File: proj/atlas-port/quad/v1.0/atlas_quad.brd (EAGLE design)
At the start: 104.1 x 95.2 mm, 110 parts, among them J11 PJ-036AH, J12 PJ-036AH, J13 5227161-9, J14 Atlas Stamp, J15 I2C-HEADER, J16 54602-908LF, J17 54602-908LF, J19 5227161-9, J20 Atlas Stamp, J21 I2C-HEADER, J4 5227161-9, J5 Atlas Stamp, J6 I2C-HEADER, J7 5227161-9, J8 Atlas Stamp, J9 I2C-HEADER, U10 ISO1540, U11 MIC4680, U12 PCA9615, U13 RM-3.33.3S, U14 ISO1540, U3 RM-3.33.3S, U4 ISO1540, U5 RM-3.33.3S, U6 ISO1540, U8 LM2937, U9 RM-3.33.3S

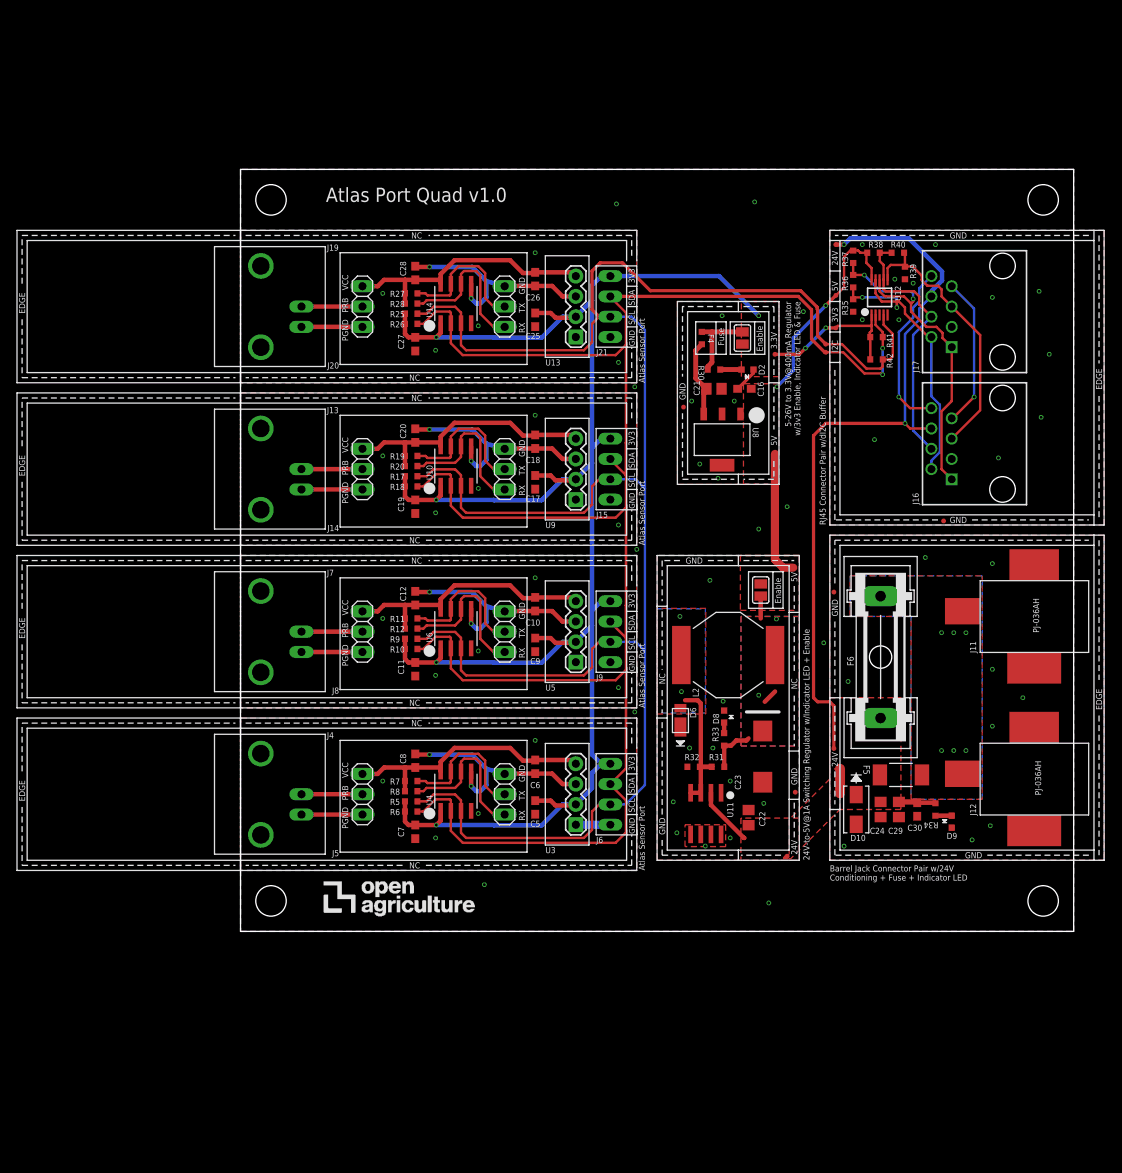
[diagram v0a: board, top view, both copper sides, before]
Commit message: added photon quad v1.0 at 90%
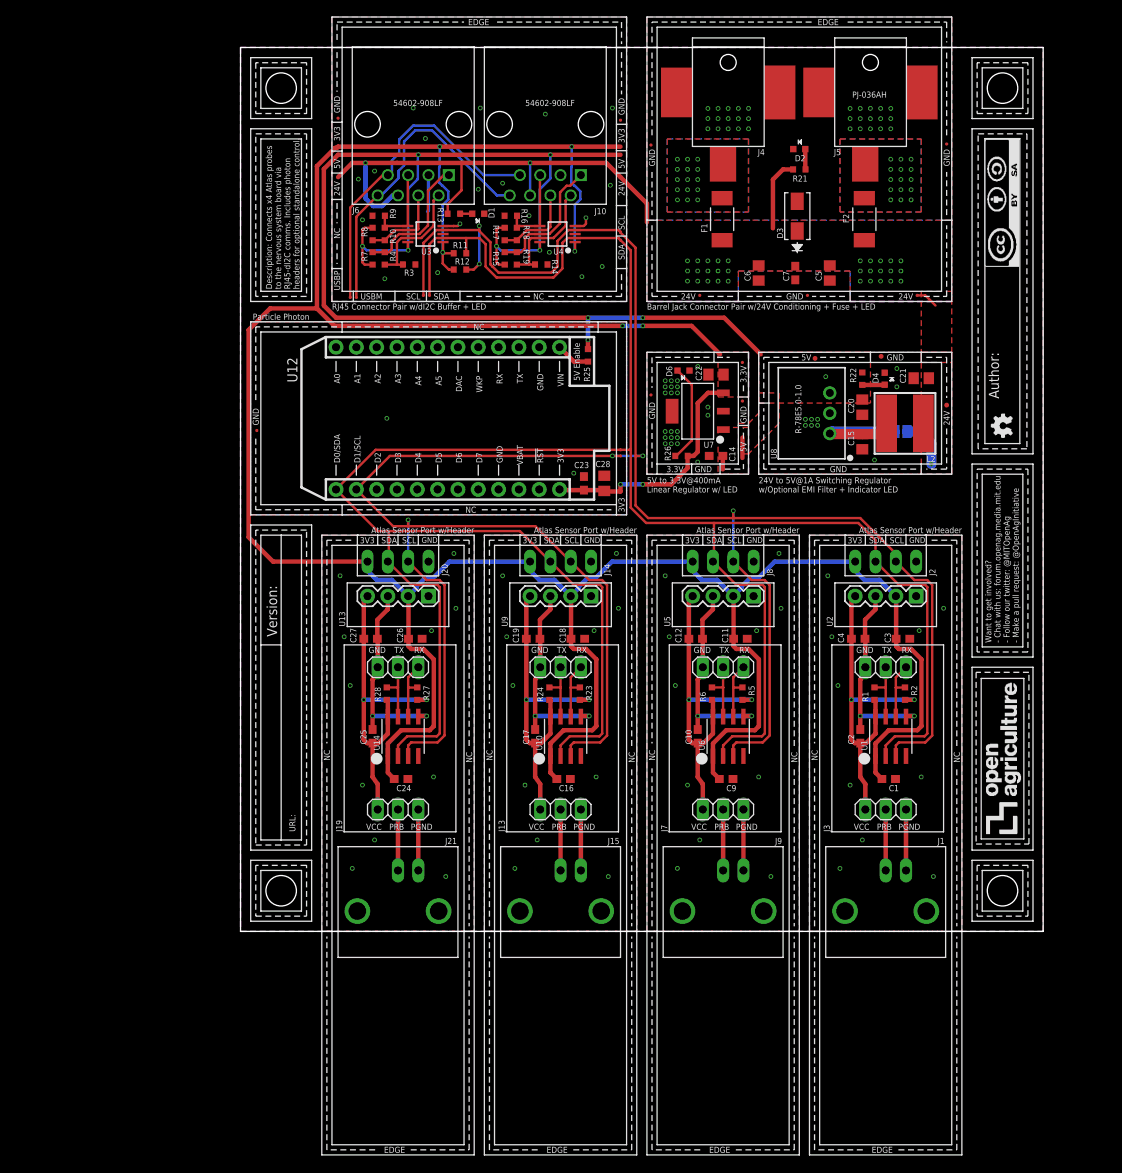
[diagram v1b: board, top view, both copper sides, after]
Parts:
- removed C29: 4.7uF, openag-capacitors:C0805
- removed C30, C8: 0.1uF, openag-capacitors:C0603
- removed D10: SMAJ26A, openag-diodes:SMA
- removed D8, D9: APT1608, openag-diodes:CHIPLED_0603
- removed F4: 0448.400MR, openag-fuses:0603
- removed F5: SST7, openag-fuses:SS
- removed F6: (no value), openag-fuses:GSH15
- removed FRAME1: (no value), openag-frames:DOCFIELD
- removed J11, J12: PJ-036AH, openag-connectors:PJ-036AH
- removed J16, J17: 54602-908LF, openag-connectors:OPENAG-V1-RJ45
- removed R20: 1K, openag-resistors:RC0603N
- removed R30, R33, R34: 100, openag-resistors:RC0603N
- removed R31: 3.01K, openag-resistors:RC0603N
- removed R32: 976 Ohm, openag-resistors:RC0603N
- removed R35, R37, R38, R39: 600, openag-resistors:RC0603N
- removed R36, R40: 120, openag-resistors:RC0603N
- removed R41, R42: 10K, openag-resistors:RC0603N
- removed SJ4: (no value), openag-connectors:SOLDERJUMPER_REFLOW_NOPASTE
- removed TP16: TPTP06R, openag-testpads:TP06R
- removed U11: MIC4680, openag-regulators:SOIC8
- added C1, C14, C2, C3, C4: 0.1uF, openag-capacitors:C0603
- added C15: 10uF, openag-capacitors:C0805
- added D1, D4: APT1608, openag-diodes:CHIPLED_0603
- added D3: SMAJ26A, openag-diodes:SMA
- added F1, F2: SSQ5, openag-fuses:SS
- added J1: 5227161-9, openag-connectors:BNC-5227161
- added J10: 54602-908LF, openag-connectors:RJ45-DI2C-USB-54602-908LF
- added J2: I2C-HEADER, openag-connectors:HEADER-I2C
- added J3: ATLAS-STAMP, openag-connectors:ATLAS-STAMP
- added R1, R2, R23, R24: 2.2k, openag-resistors:RC0603N
- added R13: 1K, openag-resistors:RC0603N
- added R14, R15, R16, R3: 600, openag-resistors:RC0603N
- added R21, R22: 100, openag-resistors:RC0603N
- added R4: 120, openag-resistors:RC0603N
- added TP19, TP20, TP28, TP29, TP30, TP31, TP32, TP4, TP5, TP58, TP6, TP7, TP71, TP72, TP73: TPTP04R, openag-testpads:TP04R
- added TP23, TP24, TP25: TPTP06R, openag-testpads:TP06R
- added U$6: TITLE, openag-frames:TITLE
- added U$8: (no value), openag-frames:LOGO-900X300
- added U1: ISO1540, openag-isolators:D8
- added U2: RM-3.33.3S, openag-isolators:RM3.33.3S-SIP4
- added U7: LM2937-3.3V, openag-regulators:MP04A
- C20, C5: value 0.1uF -> 10uF; device openag-capacitors:C0603 -> openag-capacitors:C0805
- C22: value 15uF -> 10uF
- C23: value 220uF -> 0.1uF; device openag-capacitors:CT7343 -> openag-capacitors:C0603
- C24: value 10uF -> 0.1uF; device openag-capacitors:C0805 -> openag-capacitors:C0603
- C28, C6: value 0.1uF -> 4.7uF; device openag-capacitors:C0603 -> openag-capacitors:C0805
- D6: value SBR2A40P1-7 -> APT1608; device openag-diodes:POWERDI123 -> openag-diodes:CHIPLED_0603
- J13, J19, J7: value 5227161-9 -> ATLAS-STAMP; device openag-connectors:BNC -> openag-connectors:ATLAS-STAMP
- J14, J20, J8: value Atlas Stamp -> I2C-HEADER; device openag-connectors:ATLAS-STAMP -> openag-connectors:HEADER-I2C
- J15, J21, J9: value I2C-HEADER -> 5227161-9; device openag-connectors:OPENAG-I2C-HEADER -> openag-connectors:BNC-5227161
- J4: value 5227161-9 -> PJ-036AH; device openag-connectors:BNC -> openag-connectors:BARREL-JACK-PJ-036AH
- J5: value Atlas Stamp -> PJ-036AH; device openag-connectors:ATLAS-STAMP -> openag-connectors:BARREL-JACK-PJ-036AH
- J6: value I2C-HEADER -> 54602-908LF; device openag-connectors:OPENAG-I2C-HEADER -> openag-connectors:RJ45-DI2C-USB-54602-908LF
- L2: value 68uH -> 33uH; device openag-inductors:UP2B -> openag-inductors:29333C
- R10, R18, R19: value 1K -> 120
- R11, R12: value 1K -> 10K
- R17, R7, R8, R9: value 1K -> 600
- R25: value 1K -> 0 OHM
- R26: value 1K -> 100
- R27, R28, R5, R6: value 1K -> 2.2k
- SJ1: device openag-connectors:SOLDERJUMPER_REFLOW_NOPASTE -> openag-connectors:EMI-BYPASS
- TP1, TP10, TP11, TP12, TP13, TP14, TP15, TP17, TP18, TP2, TP3, TP8, TP9: value TPTP06R -> TPTP04R; device openag-testpads:TP06R -> openag-testpads:TP04R
- U$1, U$2, U$3, U$4: device openag-frames:OPENAG-CORNER-MOUNTING-HOLE -> openag-frames:CORNER-150
- U$5: value (none) -> AUTHOR; device openag-frames:OPENAG-LOGO-750-MIL -> openag-frames:AUTHOR
- U12: value PCA9615 -> PHOTONH; device openag-buffers:SOP50P490X110-10N -> openag-microcontrollers:PHOTON
- U13, U5, U9: device openag-isolators:SIP4 -> openag-isolators:RM3.33.3S-SIP4
- U3: value RM-3.33.3S -> PCA9615; device openag-isolators:SIP4 -> openag-buffers:SOP50P490X110-10N
- U4: value ISO1540 -> PCA9615; device openag-isolators:D8 -> openag-buffers:SOP50P490X110-10N
- U8: value LM2937 -> R-78E5.0-1.0; device openag-regulators:MP04A -> openag-regulators:R-78E5.0-1.0
- moved U$2 136.7 mm to (95.2, 105.4), turned to 180 degrees
- moved U$1 125.8 mm to (95.2, 5.08), turned to 90 degrees
- moved U$5 105.6 mm to (99.1, 59.7), turned to 90 degrees
- moved J4 99.8 mm to (61.0, 98.1), turned to 270 degrees
- moved J5 97.7 mm to (78.7, 98.1), turned to 270 degrees
- moved U$4 96.3 mm to (5.08, 105.4), turned to 270 degrees
- moved U$3 95.3 mm to (5.08, 5.08), turned to 0 degrees
- moved TP10 90.1 mm to (47.5, 97.1)
- moved J6 87.5 mm to (21.6, 100.9), turned to 180 degrees
- moved C7 84.5 mm to (69.3, 82.3)
- moved TP9 83.6 mm to (47.5, 98.1)
- moved TP12 82.9 mm to (47.5, 101.4), turned to 270 degrees
- moved J21 80.3 mm to (19.7, 2.54), turned to 180 degrees
- moved C5 76.3 mm to (73.7, 82.3)
- moved U3 76.2 mm to (23.1, 87.2), turned to 180 degrees
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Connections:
- removed net 24V_IN: F5.1, F6.1, J11.1, J12.1
- removed net DSCLM: J16.DSCLM(5), J17.DSCLM(5), R39.2, R40.1, U12.6
- removed net DSCLP: J16.DSCLP(4), J17.DSCLP(4), R38.1, R40.2, U12.7
- removed net DSDAM: J16.DSDAM(2), J17.DSDAM(2), R35.1, R36.2, U12.9
- removed net DSDAP: J16.DSDAP(1), J17.DSDAP(1), R36.1, R37.2, U12.8
- removed net N$27: D8.A, R33.1
- removed net N$45: C23.+, L2.2, R31.2, R33.2, SJ4.1
- removed net N$46: D9.A, R34.1
- removed net REG_3V3_400MA: F4.2, R30.2, SJ1.1
- new net 24V_EMI: C15.1, L2.2, SJ1.2, U8.1
- new net 24V_IN1: F2.1, J5.1
- new net 24V_IN2: F1.1, J4.1
- new net DSCLM_1: J6.DSCLM(5), R10.1, R9.2, U3.6
- new net DSCLM_2: J10.DSCLM(5), R16.2, R18.1, U4.6
- new net DSCLP_1: J6.DSCLP(4), R10.2, R8.1, U3.7
- new net DSCLP_2: J10.DSCLP(4), R17.1, R18.2, U4.7
- new net DSDAM_1: J6.DSDAM(2), R3.1, R4.2, U3.9
- new net DSDAM_2: J10.DSDAM(2), R14.1, R19.2, U4.9
- new net DSDAP_1: J6.DSDAP(1), R4.1, R7.2, U3.8
- new net DSDAP_3: J10.DSDAP(1), R15.2, R19.1, U4.8
- new net N$4: R25.2, U12.1
- new net N$5: D1.A, R13.1
- new net VBAT: U12.22
- net +24V: now also C21.1, C5.1, C6.1, C7.1, D3.1, F1.2, F2.2, J10.24V(6), J6.24V(6), L2.1, R13.2, R21.2, SJ1.1, TP11.1, TP17.1, TP20.1, TP24.TP, TP4.1; no longer C22.1, C24.1, C29.1, C30.1, D10.1, F5.2, F6.2, J16.24V(6), J17.24V(6), R34.2, TP10.TP, TP12.TP, TP18.TP, U11.2
- net +3V3: now also C1.1, C16.1, C18.1, C22.1, C23.1, C24.1, C26.1, C28.1, C3.1, J14.3V3, J2.3V3, J20.3V3, J8.3V3, R11.2, R12.2, TP1.1, TP28.1, TP31.1, TP71.1, TP9.1, U1.1, U12.24, U2.2, U3.1, U7.3; no longer C17.1, C19.1, C25.1, C27.1, C5.1, C7.1, J15.3V3, J21.3V3, J6.3V3, J9.3V3, R10.2, R17.2, R18.2, R25.2, R41.2, R42.2, R5.2, R6.2, R9.2, SJ1.2, TP15.TP, TP3.TP, U12.1, U3.2
- net +5V: now also C14.1, C20.1, R15.1, R17.2, R22.2, R25.1, R7.1, R8.2, TP10.1, TP2.1, TP23.TP, TP29.1, U3.10, U4.10, U7.1, U8.3; no longer C16.1, R37.1, R38.2, SJ4.2, TP17.TP, TP2.TP, TP8.TP, U12.10, U8.1
- net GND: now also C1.2, C14.2, C15.2, C18.2, C20.2, C23.2, C26.2, C28.2, C3.2, C6.2, D1.C, D3.2, D4.C, D6.C, J10.GND(3), J14.GND, J2.GND, J20.GND, J4.2, J4.3, J5.2, J5.3, J6.GND(3), J8.GND, R14.2, R16.1, R3.2, R9.1, TP12.1, TP15.1, TP18.1, TP19.1, TP25.TP, TP3.1, TP30.1, TP32.1, TP72.1, U1.4, U12.2, U12.21, U2.1, U3.5, U4.5, U7.2, U7.4; no longer C17.2, C19.2, C23.-, C25.2, C27.2, C29.2, C30.2, D10.2, D6.-, D8.C, D9.C, J11.2, J11.3, J12.2, J12.3, J15.GND, J16.GND(3), J17.GND(3), J21.GND, J6.GND, J9.GND, R32.1, R35.2, R39.1, TP1.TP, TP11.TP, TP16.TP, TP9.TP, U11.1, U11.5, U11.6, U11.7, U11.8, U12.5, U3.1, U4.4, U8.4
- net ISO_3V3_1: now also C2.1, C4.1, J3.4, R1.2, R2.2, U1.8, U2.4; no longer C6.1, C8.1, J5.4, R7.2, R8.2, U3.4, U4.8
- net ISO_3V3_2: now also J7.4, R5.2, R6.2; no longer J8.4, R11.2, R12.2
- net ISO_3V3_3: now also C17.1, C19.1, J13.4, R23.2, R24.2; no longer C18.1, C20.1, J14.4, R19.2, R20.2
- net ISO_3V3_4: now also C25.1, C27.1, J19.4; no longer C26.1, C28.1, J20.4
- net ISO_GND_1: now also C2.2, C4.2, J3.3, U1.5, U2.3; no longer C6.2, C8.2, J5.3, U3.3, U4.5
- net ISO_GND_2: now also J7.3; no longer J8.3
- net ISO_GND_3: now also C17.2, C19.2, J13.3; no longer C18.2, C20.2, J14.3
- net ISO_GND_4: now also C25.2, C27.2, J19.3; no longer C26.2, C28.2, J20.3
- net ISO_SCL_1: now also J3.1, R2.1, U1.6; no longer J5.1, R8.1, U4.6
- net ISO_SCL_2: now also J7.1, R5.1; no longer J8.1, R12.1
- net ISO_SCL_3: now also J13.1, R23.1; no longer J14.1, R20.1
- net ISO_SCL_4: now also J19.1, R27.1; no longer J20.1, R28.1
- net ISO_SDA_1: now also J3.2, R1.1, U1.7; no longer J5.2, R7.1, U4.7
- net ISO_SDA_2: now also J7.2, R6.1; no longer J8.2, R11.1
- net ISO_SDA_3: now also J13.2, R24.1; no longer J14.2, R19.1
- net ISO_SDA_4: now also J19.2, R28.1; no longer J20.2, R27.1
- net N$11: now also D6.A, R26.1; no longer D6.+, L2.1, R31.1, R32.2, U11.3, U11.4
- net N$6: now also R21.1; no longer R30.1
- net N$8: now also D4.A, R22.1; no longer C21.1, F4.1, U8.3
- net PGND_1: now also J1.GND, J3.6; no longer J4.GND, J5.6
- net PGND_2: now also J7.6, J9.GND; no longer J7.GND, J8.6
- net PGND_3: now also J13.6, J15.GND; no longer J13.GND, J14.6
- net PGND_4: now also J19.6, J21.GND; no longer J19.GND, J20.6
- net PRB_1: now also J1.S, J3.5; no longer J4.S, J5.5
- net PRB_2: now also J7.5, J9.S; no longer J7.S, J8.5
- net PRB_3: now also J13.5, J15.S; no longer J13.S, J14.5
- net PRB_4: now also J19.5, J21.S; no longer J19.S, J20.5
- net SCL: now also J14.SCL, J2.SCL, J20.SCL, J8.SCL, R12.1, TP13.1, TP58.1, TP6.1, U1.3, U12.14, U3.4, U4.4; no longer J15.SCL, J21.SCL, J6.SCL, J9.SCL, R17.1, R25.1, R42.1, R5.1, R9.1, TP13.TP, U12.4, U4.3
- net SDA: now also J14.SDA, J2.SDA, J20.SDA, J8.SDA, R11.1, TP14.1, TP5.1, TP73.1, U1.2, U12.13, U3.2; no longer J15.SDA, J21.SDA, J6.SDA, J9.SDA, R10.1, R18.1, R26.1, R41.1, R6.1, TP14.TP, U12.2
- net USBM: now also J10.USBM(8), J6.USBM(8), TP8.1; no longer J16.USBM(8), J17.USBM(8)
- net USBP: now also J10.USBP(7), J6.USBP(7), TP7.1; no longer J16.USBP(7), J17.USBP(7)
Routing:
- net +3V3: track 255.2 -> 428.3 mm, vias 7 -> 8
- net +5V: track 42.7 -> 171.9 mm, vias 2 -> 9
- net SDA: track 250.1 -> 320.4 mm, vias 2 -> 0
- net SCL: track 263.9 -> 325.3 mm, vias 0 -> 6
- net DSDAP: track 43.2 -> 0.00 mm, vias 2 -> 0
- net DSDAM: track 38.1 -> 0.00 mm, vias 2 -> 0
- net DSCLM: track 33.9 -> 0.00 mm
- net DSCLP: track 32.7 -> 0.00 mm
- net +24V: track 108.5 -> 82.7 mm, vias 2 -> 33
- net USBP: track 18.9 -> 41.0 mm, vias 1 -> 0
- net USBM: track 21.4 -> 39.4 mm, vias 1 -> 0
- net DSDAP_1: track 0.00 -> 16.7 mm
- net DSDAP_3: track 0.00 -> 16.5 mm
- net 24V_EMI: track 0.00 -> 15.9 mm
- net DSDAM_2: track 0.00 -> 14.7 mm
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- added copper zone on layer 16, net +24V
- added copper zone on layer 1, net 24V_IN1
- added copper zone on layer 16, net 24V_IN1
- added copper zone on layer 1, net 24V_IN2
- added copper zone on layer 16, net 24V_IN2
- removed copper zone on layer 1, net 24V_IN
- removed copper zone on layer 16, net 24V_IN
- removed copper zone on layer 1, net N$11
- removed copper zone on layer 16, net N$11
- removed copper zone on layer 1, net N$45
- removed copper zone on layer 16, net N$45
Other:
- board size 104.1 x 95.2 mm -> 100.3 x 110.5 mm
- board text added: "24V to 5V@1A Switching Regulator w/Optional EMI Filter + Indicator LED"
- board text added: "5V Enable"
- board text added: "5V to 3.3V@400mA Linear Regulator w/ LED"
- board text added: "Atlas Sensor Port w/Header"
- board text added: "Barrel Jack Connector Pair w/24V Conditioning + Fuse + LED"
- board text added: "Description: Connects x4 Atlas probes to the nervous system board via RJ45-dI2C comms. Includes photon headers for optional standalone control."
- board text added: "Particle Photon"
- board text added: "RJ45 Connector Pair w/dI2C Buffer + LED"
- board text added: "SCL"
- board text added: "SDA"
- board text added: "USBM"
- board text added: "USBP"
- board text added: "Want to get involved? - Chat with us: forum.openag.media.mit.edu - Follow our twitter: @MITOpenAg - Make a pull request: @OpenAgInitiative"
- board text removed: "24V-to-5V@1A Switching Regulator w/Indicator LED + Enable"
- board text removed: "5-26V to 3.3V@400mA Regulator w/3v3 Enable, Indicator LED & Fuse"
- board text removed: "Atlas Port Quad v1.0"
- board text removed: "Atlas Sensor Port"
- board text removed: "Barrel Jack Connector Pair w/24V Conditioning + Fuse + Indicator LED"
- board text removed: "Enable"
- board text removed: "Fuse"
- board text removed: "I2C"
- board text removed: "RJ45 Connector Pair w/dI2C Buffer"
